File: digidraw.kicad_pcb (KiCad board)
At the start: 2 copper layers, 100 x 100 mm, 152 parts, among them CON1 SN49B12B, J1 USB_B_Micro, J10 USB_A, J11 Conn_02x05_Odd_Even, J12 Conn_01x03_Male, J13 Conn_01x04_Male, J2 Barrel_Jack, J3 Conn_02x05_Odd_Even, J4 Conn_01x06_Male, J5 Conn_01x05_Male, J6 Conn_01x04_Male, J7 Conn_01x15_Female, J8 Conn_01x04_Male, J9 Conn_01x05_Male, Q1 FDD5614P, SW1 SW_Push_Dual, SW2 SW_Push_Dual, SW3 SW_Push_Dual, SW4 SW_Push_Dual, SW5 SW_Push_Dual, SW6 SW_Push_Dual, U1 TPS63070RNMR, U2 V7803-1500R, U3 STM32F051R8T6, U4 CAT24C256, U5 STM32F407VGT6, U6 PCM5102, U7 STMPS2141STR, U8 LM317KCS, U9 USBLC6-2SC6, Y1 8MHz, Y2 8MHz

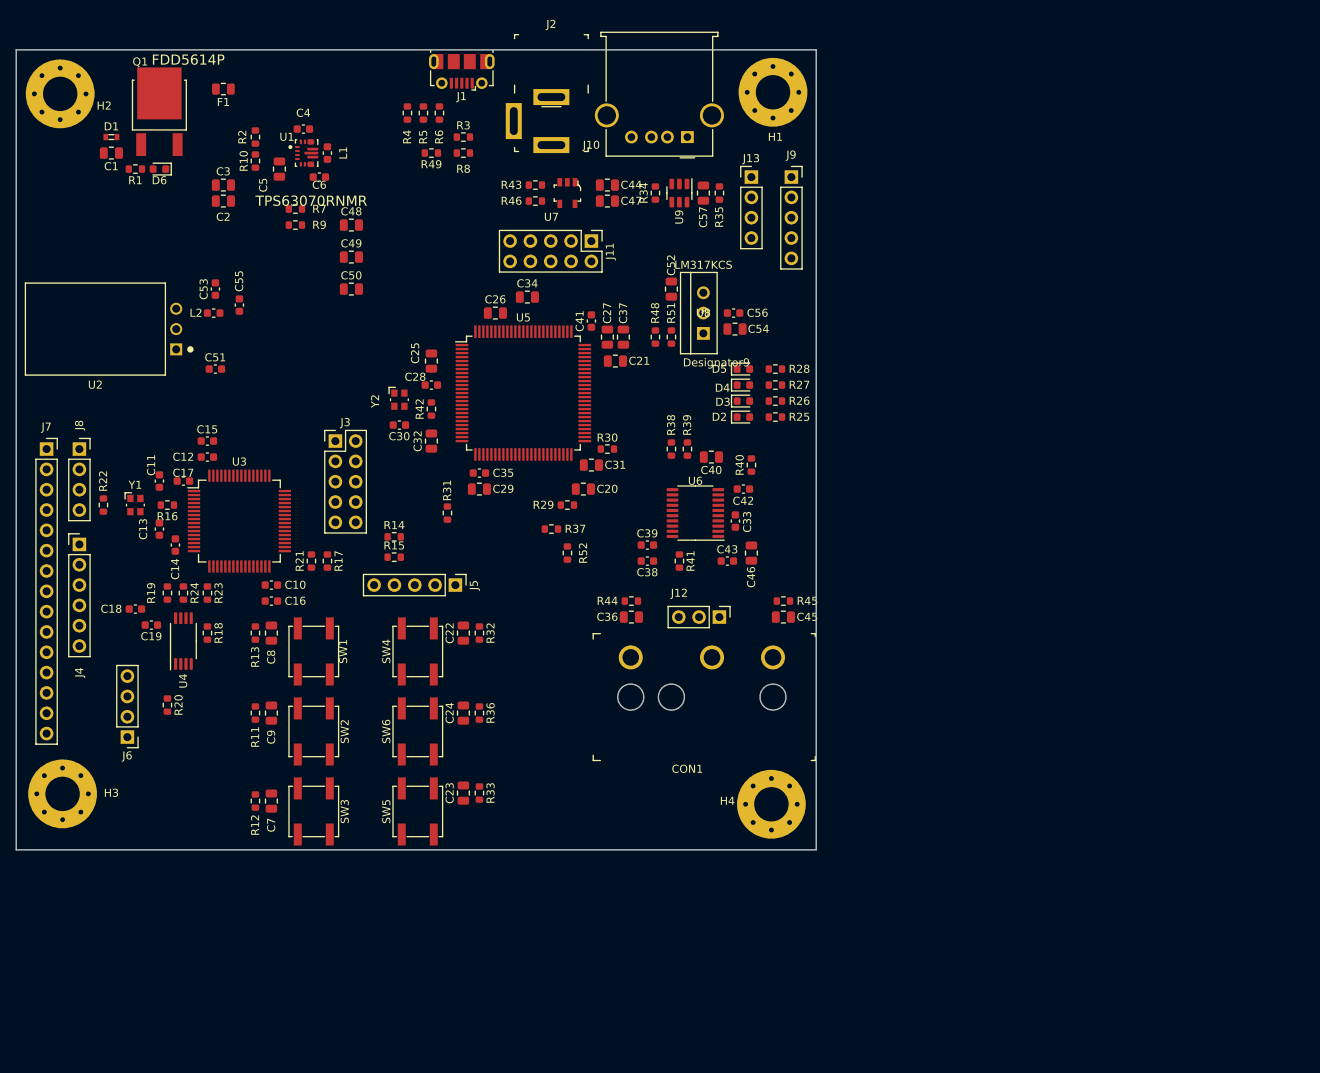
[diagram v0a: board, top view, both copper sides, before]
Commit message: Replace components
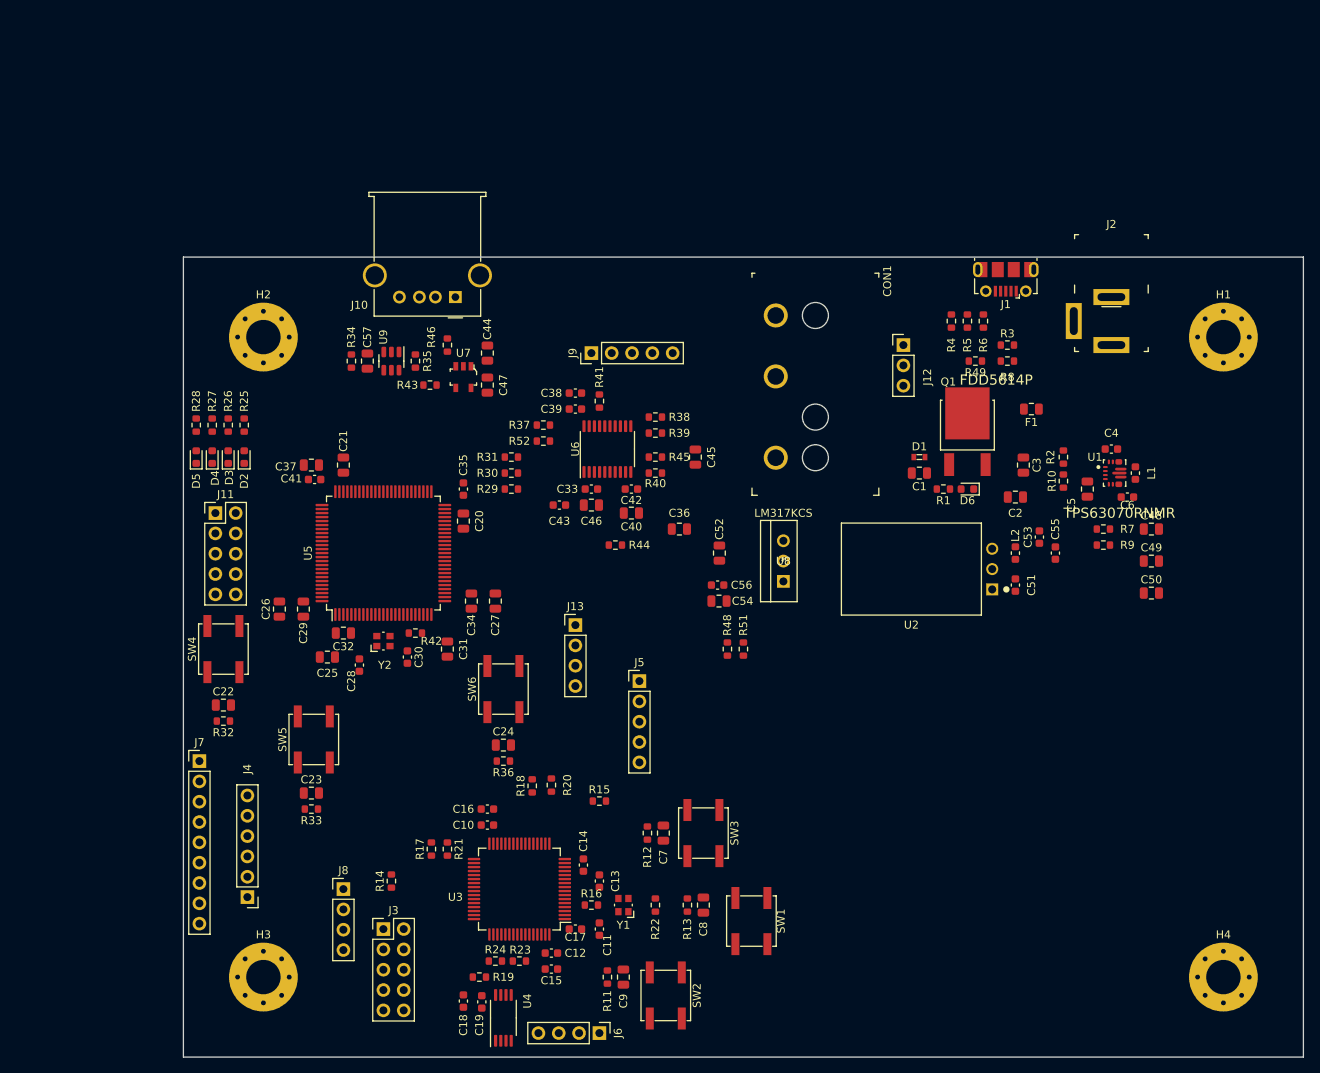
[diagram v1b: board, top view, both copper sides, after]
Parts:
- J7: value Conn_01x15_Female -> Conn_01x09_Male; footprint Connector_PinSocket_2.54mm:PinSocket_1x15_P2.54mm_Vertical -> Connector_PinHeader_2.54mm:PinHeader_1x09_P2.54mm_Vertical
- J8: footprint Connector_PinSocket_2.54mm:PinSocket_1x04_P2.54mm_Vertical -> Connector_PinHeader_2.54mm:PinHeader_1x04_P2.54mm_Vertical
- J9: footprint Connector_PinSocket_2.54mm:PinSocket_1x05_P2.54mm_Vertical -> Connector_PinHeader_2.54mm:PinHeader_1x05_P2.54mm_Vertical
- moved C1 108.6 mm to (151.0, 91.0)
- moved C4 108.6 mm to (175.0, 88.0)
- moved C5 108.6 mm to (172.0, 93.0)
- moved C6 108.6 mm to (177.0, 94.0)
- moved D1 108.6 mm to (151.0, 89.0)
- moved D6 108.6 mm to (157.0, 93.0)
- moved F1 108.6 mm to (165.0, 83.0)
- moved L1 108.6 mm to (178.0, 91.0)
- moved Q1 108.6 mm to (157.0, 85.0)
- moved R1 108.6 mm to (154.0, 93.0)
- moved R10 108.6 mm to (169.0, 92.0)
- moved R2 108.6 mm to (169.0, 89.0)
- moved R7 108.6 mm to (174.0, 98.0)
- moved R9 108.6 mm to (174.0, 100.0)
- moved U1 108.6 mm to (175.4, 91.0)
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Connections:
- J4 pad 2: /user_io/RA8875_MISO -> /user_io/RA8875_NSS
- J4 pad 4: /user_io/RA8875_SCK -> /user_io/RA8875_MISO
- J4 pad 5: /user_io/RA8875_NSS -> /user_io/RA8875_SCK
- J7 pad 3: Net-(J7-Pad3) -> /user_io/RA8875_SCK
- J7 pad 4: Net-(J7-Pad4) -> /user_io/RA8875_MISO
- J7 pad 5: /user_io/RA8875_SCK -> /user_io/RA8875_MOSI
- J7 pad 6: /user_io/RA8875_MISO -> /user_io/RA8875_NSS
- J7 pad 7: /user_io/RA8875_MOSI -> /user_io/RA8875_NRST
- J7 pad 8: /user_io/RA8875_NSS -> /user_io/RA8875_WAIT
- J7 pad 9: /user_io/RA8875_NRST -> /user_io/RA8875_INT
- J9 pad 2: /midi_dac/I2S_SD -> /midi_dac/I2S_WS
- J9 pad 3: /midi_dac/I2S_CK -> /midi_dac/I2S_SD
- J9 pad 4: /midi_dac/I2S_WS -> /midi_dac/I2S_CK
- U5 pad 15: /midi_dac/USB_VBUS_EN -> Net-(U5-Pad15)
- U5 pad 18: Net-(R31-Pad2) -> Net-(U5-Pad18)
- U5 pad 23: /midi_dac/GPIO_EXTI0 -> /midi_dac/UART4_TX
- U5 pad 31: Net-(U5-Pad31) -> /midi_dac/SPI_INT
- U5 pad 54: Net-(U5-Pad54) -> Net-(R31-Pad2)
- U5 pad 69: Net-(U5-Pad69) -> /midi_dac/USB_VBUS_EN
- U5 pad 78: /midi_dac/UART4_TX -> Net-(U5-Pad78)
- U5 pad 90: /midi_dac/SPI_INT -> Net-(U5-Pad90)
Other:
- board size 100 x 100 mm -> 140 x 100 mm
